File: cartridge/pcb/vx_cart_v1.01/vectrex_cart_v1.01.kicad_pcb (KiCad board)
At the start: 2 copper layers, 47 x 47.2 mm, 7 parts, among them J1 Vectrex Cartridge Connector, U1 27C256

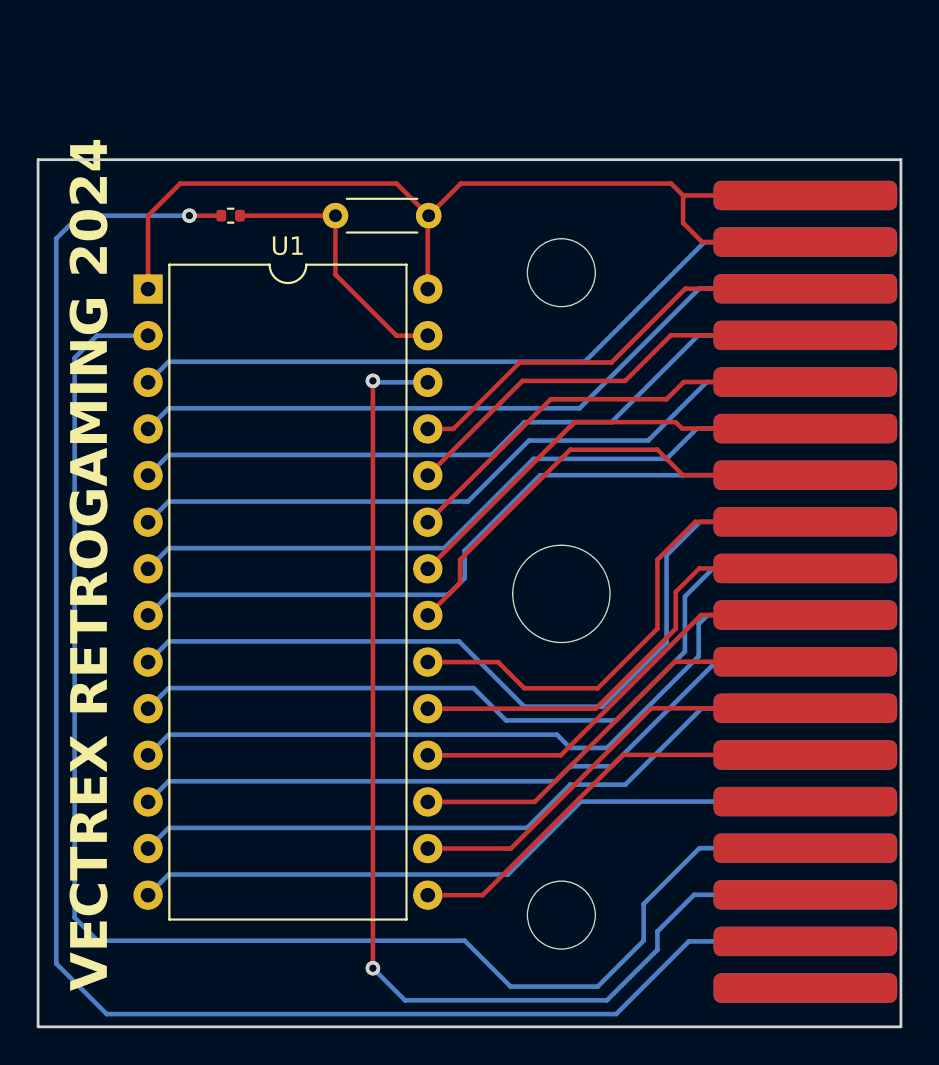
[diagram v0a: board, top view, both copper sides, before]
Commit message: Cart PCB v1.01
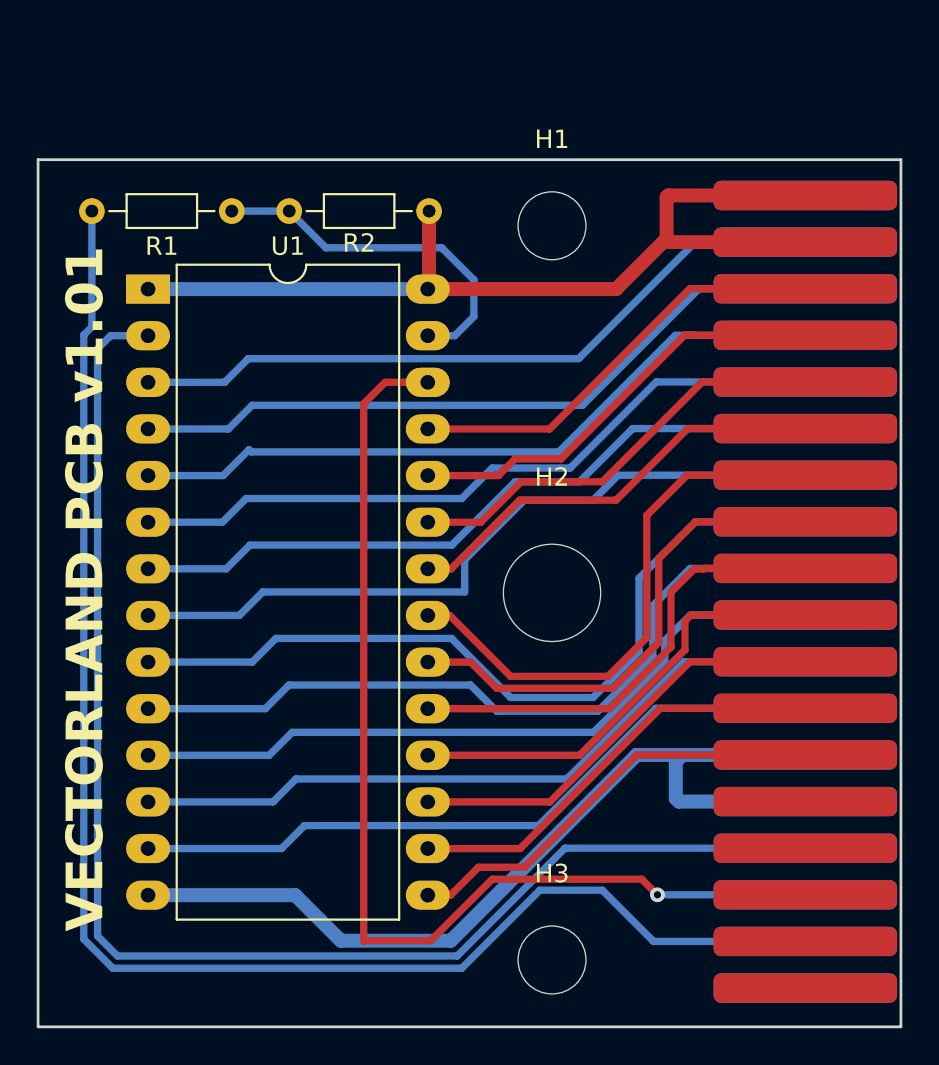
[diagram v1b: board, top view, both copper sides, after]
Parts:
- added G***: LOGO, LogoVx:vx3, B.Cu at (102.8, 69.5)
- R1: value SP -> 0R; footprint Resistor_SMD:R_0402_1005Metric -> Resistor_THT:R_Axial_DIN0204_L3.6mm_D1.6mm_P7.62mm_Horizontal
- R2: footprint Resistor_THT:R_Axial_DIN0204_L3.6mm_D1.6mm_P5.08mm_Horizontal -> Resistor_THT:R_Axial_DIN0204_L3.6mm_D1.6mm_P7.62mm_Horizontal
- U1: footprint Package_DIP:DIP-28_W15.24mm -> Package_DIP:DIP-28_W15.24mm_LongPads
- moved H1 2.61 mm to (117.0, 48.0)
- moved R2 2.53 mm to (102.7, 47.2)
- moved H3 2.50 mm to (117.0, 88.0)
- moved H2 0.51 mm to (117.0, 68.0)
- moved R1 0.26 mm to (99.6, 47.2)
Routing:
- net A14: track 88.6 -> 78.7 mm, vias 1 -> 0
- net GND: track 33.9 -> 42.7 mm
- net Net-(U1-A14): track 14.8 -> 19.7 mm
- net A10: track 21.6 -> 26.4 mm
- net A12: track 76.7 -> 72.5 mm
- net VCC: track 46.9 -> 43.2 mm
- net A13: track 58.3 -> 55.0 mm, vias 2 -> 1
- net D0: track 36.6 -> 35.6 mm
- net D6: track 19.7 -> 20.7 mm
- net A1: track 40.7 -> 40.0 mm
- net D7: track 20.9 -> 21.5 mm
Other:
- board text added: "VECTORLAND PCB v1.01"
- board text removed: "VECTREX RETROGAMING 2024"
